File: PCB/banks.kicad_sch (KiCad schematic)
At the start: 50 parts, among them U1 XC7A50T-FGG484, Y3 100MHz

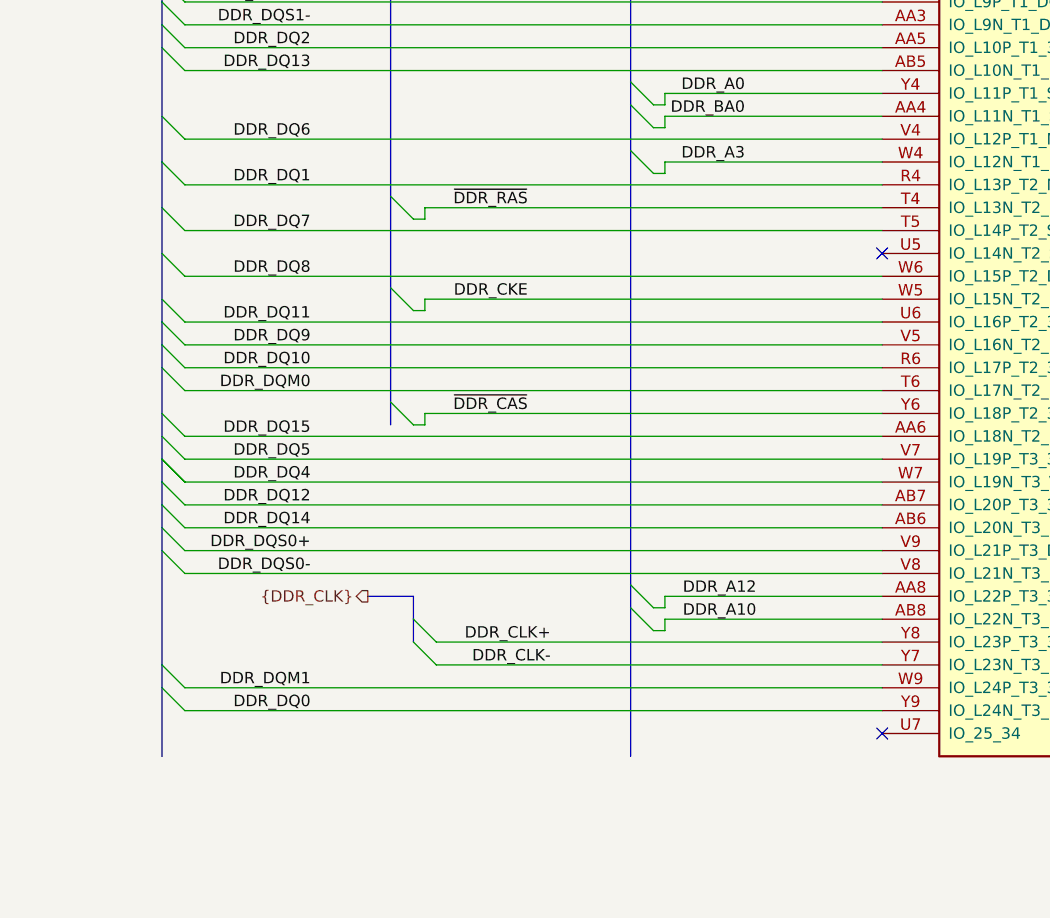
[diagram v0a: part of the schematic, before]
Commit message: finally routed a little mischevious DQ3
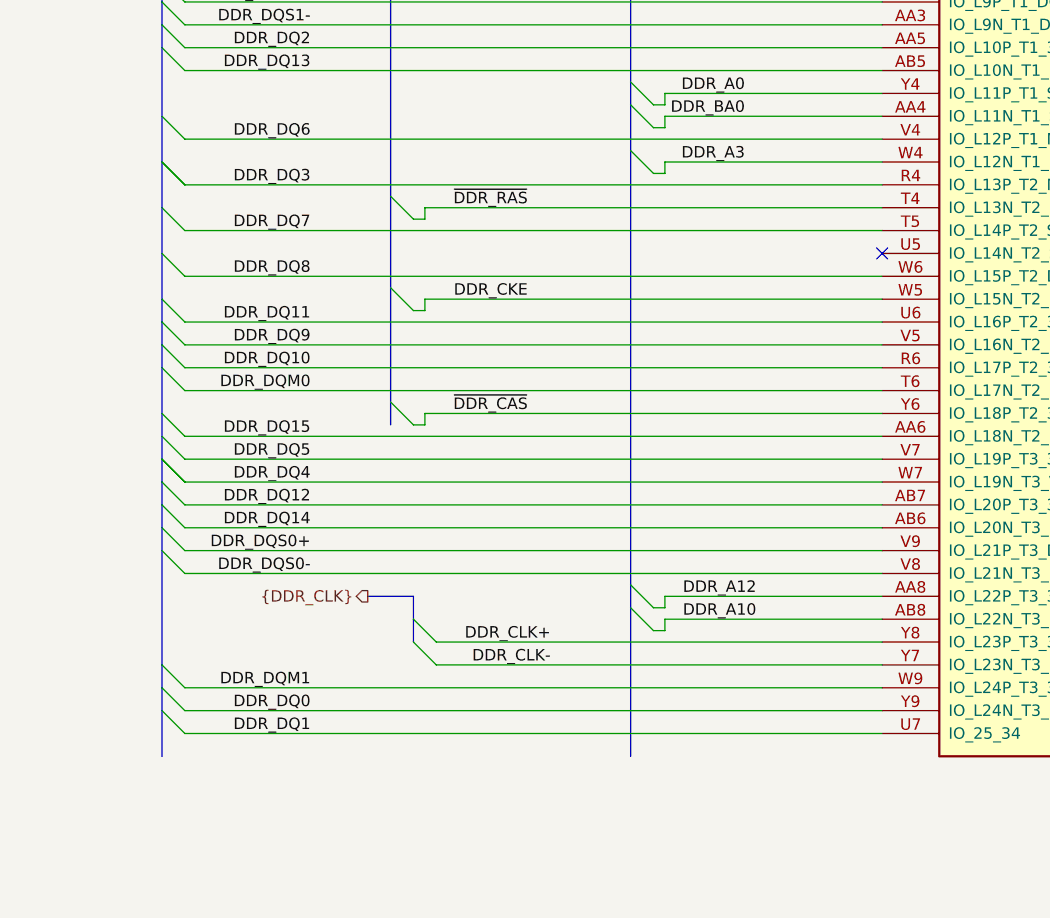
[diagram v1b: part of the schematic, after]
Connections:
- net DDR_DQ1: now also U1.U7 (IO_25_34); no longer U1.R4 (IO_L13P_T2_MRCC_34)
- new net DDR_DQ3: U1.R4 (IO_L13P_T2_MRCC_34)
- no-connect marks 14 -> 13
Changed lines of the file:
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@@
 	)
 	(no_connect
-		(at 702.31 214.63)
-	)
-	(no_connect
 		(at 702.31 100.33)
 	)
@@
 	)
 	(bus_entry
+		(at 622.3 151.13)
+		(size 2.54 2.54)
+		(stroke
+			(width 0)
+			(type default)
+		)
+	)
+	(bus_entry
 		(at 622.3 209.55)
 		(size 2.54 2.54)
@@
 	)
 	(bus_entry
+		(at 622.3 212.09)
+		(size 2.54 2.54)
+		(stroke
+			(width 0)
+			(type default)
+		)
+	)
+	(bus_entry
 		(at 622.3 194.31)
 		(size 2.54 2.54)
@@
 		)
 	)
+	(bus
+		(pts
+			(xy 622.3 212.09) (xy 622.3 217.17)
+		)
+		(stroke
+			(width 0)
+			(type default)
+		)
+	)
 	(wire
 		(pts
@@
 	(wire
 		(pts
+			(xy 624.84 153.67) (xy 702.31 153.67)
+		)
+		(stroke
+			(width 0)
+			(type default)
+		)
+	)
+	(wire
+		(pts
 			(xy 712.47 46.99) (xy 712.47 49.53)
 		)
@@
 	(bus
 		(pts
-			(xy 622.3 209.55) (xy 622.3 217.17)
+			(xy 622.3 209.55) (xy 622.3 212.09)
 		)
 		(stroke
@@
 	(wire
 		(pts
+			(xy 624.84 214.63) (xy 702.31 214.63)
+		)
+		(stroke
+			(width 0)
+			(type default)
+		)
+	)
+	(wire
+		(pts
 			(xy 802.64 49.53) (xy 810.26 49.53)
 		)
@@
 	(wire
 		(pts
-			(xy 624.84 153.67) (xy 702.31 153.67)
-		)
-		(stroke
-			(width 0)
-			(type default)
-		)
-	)
-	(wire
-		(pts
 			(xy 345.44 68.58) (xy 345.44 69.85)
 		)
@@
 		)
 	)
-	(label "DDR_DQ1"
-		(at 638.81 153.67 180)
-		(effects
-			(font
-				(size 1.27 1.27)
-			)
-			(justify right bottom)
-		)
-	)
 	(label "QSPI_DQ3"
 		(at 140.97 100.33 180)
@@
 		)
 	)
+	(label "DDR_DQ1"
+		(at 638.81 214.63 180)
+		(effects
+			(font
+				(size 1.27 1.27)
+			)
+			(justify right bottom)
+		)
+	)
 	(label "DDR_A4"
 		(at 687.07 97.79 180)
@@
 		(effects
 			(font
+				(size 1.27 1.27)
+			)
+			(justify right bottom)
+		)
+	)
+	(label "DDR_DQ3"
+		(at 638.81 153.67 180)
+		(effects
+			(font
